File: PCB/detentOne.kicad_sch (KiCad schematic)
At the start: 8 parts, among them SW7 C92589, SW8 C92589, U3 ESP32-S3-WROOM-1(N16R8)

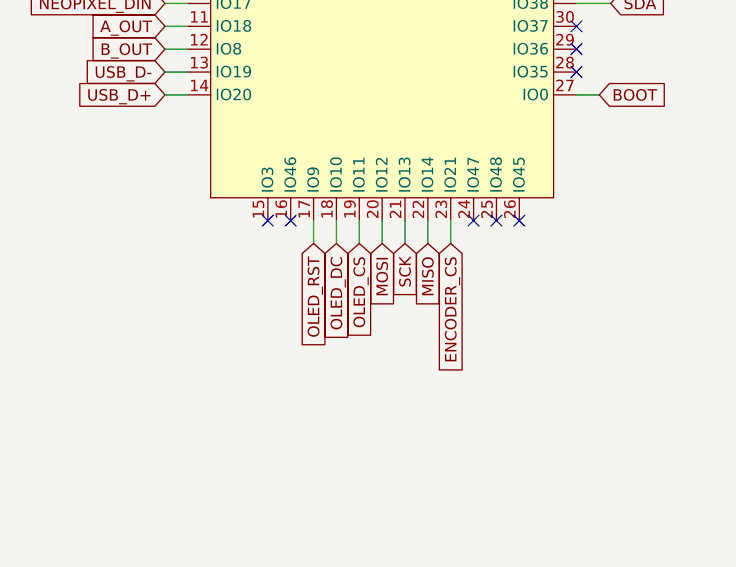
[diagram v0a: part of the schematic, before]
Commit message: PCB traced
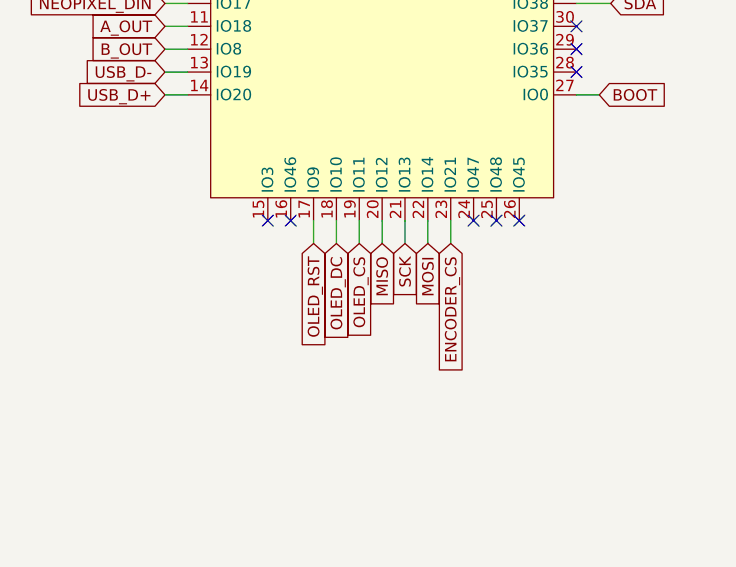
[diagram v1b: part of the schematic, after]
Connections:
- net MISO: now also U3.20 (IO12); no longer U3.22 (IO14)
- net MOSI: now also U3.22 (IO14); no longer U3.20 (IO12)
